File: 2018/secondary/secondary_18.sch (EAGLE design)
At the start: 35 parts, among them Q1 BUZ11, Q2 BUZ11

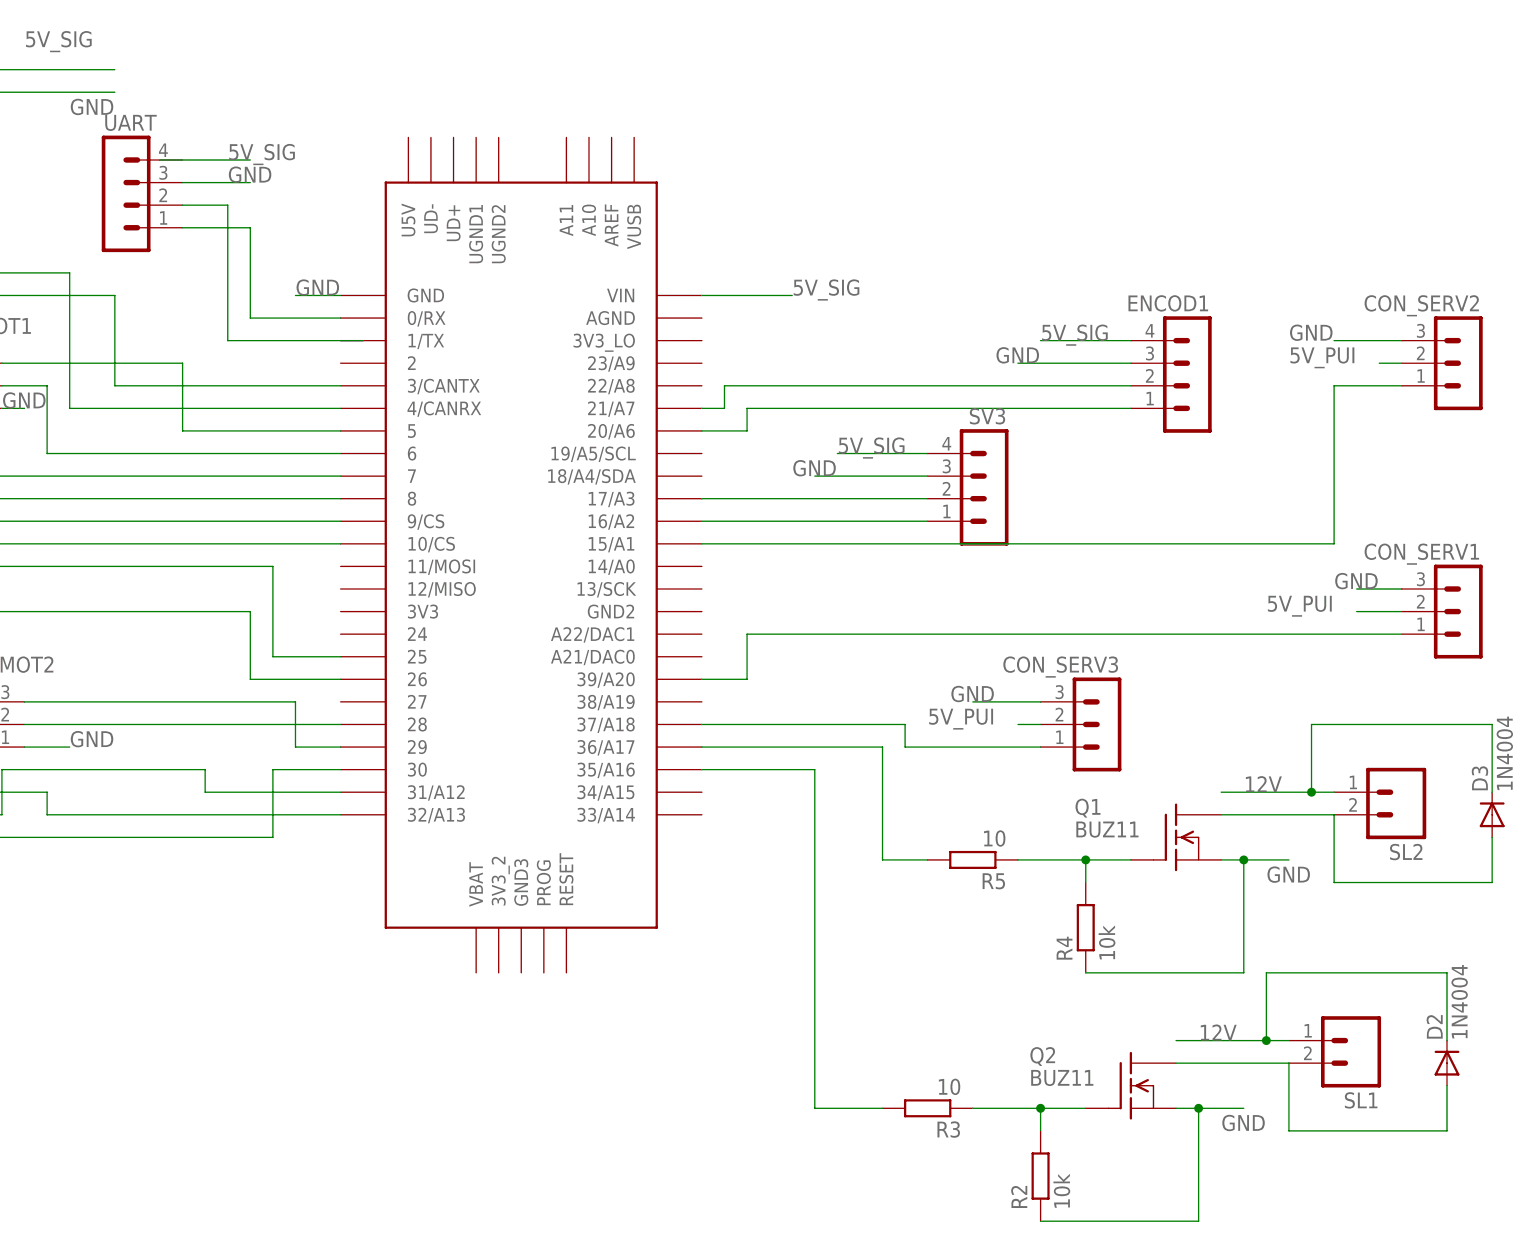
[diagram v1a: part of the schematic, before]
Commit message: [Secondary] Adds the board.
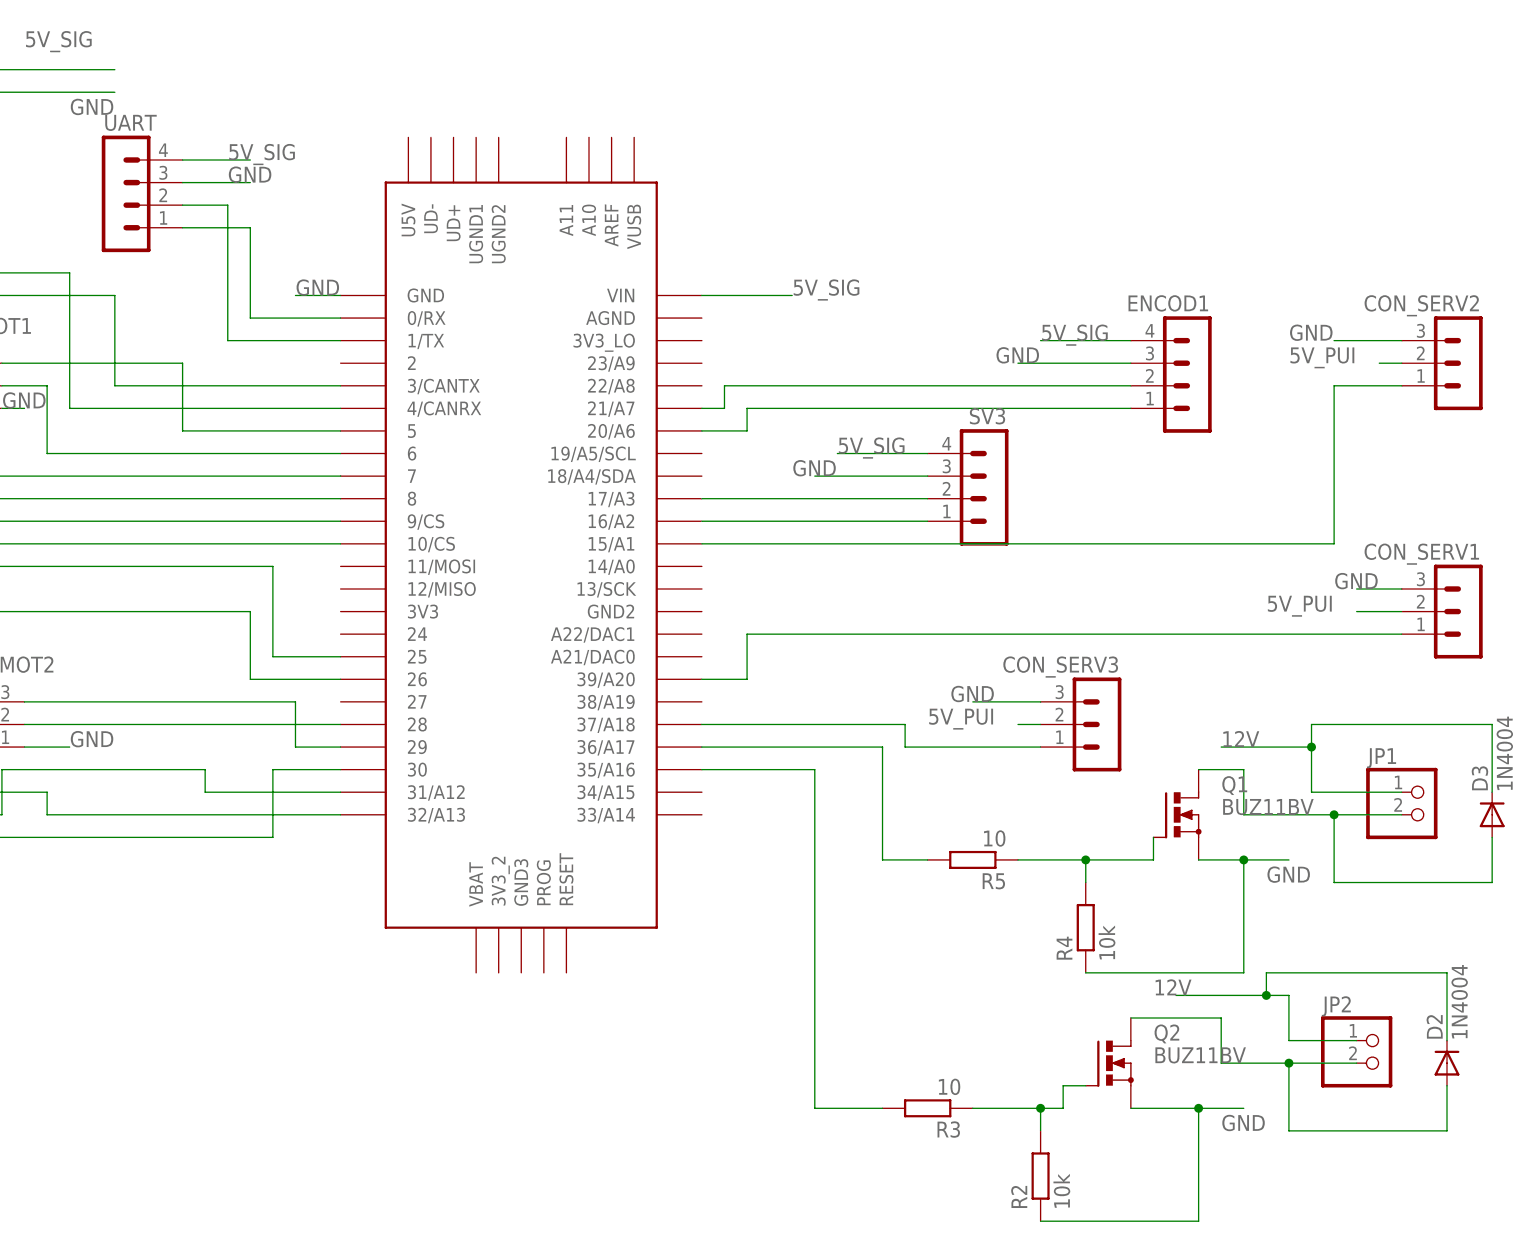
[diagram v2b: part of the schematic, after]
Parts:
- removed SL1, SL2: (no value), con-amp-quick:MA02
- added JP1, JP2: (no value), pinhead:PINHD-1X2
- Q1, Q2: value BUZ11 -> BUZ11BV; device transistor-fet:BUZ11 -> transistor-power:BUZ11BV
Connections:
- net 12V: now also JP1.1, JP2.1; no longer SL1.1, SL2.1
- net 5V_SIG: now also UART.4
- net N$12: now also JP1.2; no longer SL2.2
- net N$26: now also U$1.1/TX
- net N$8: now also JP2.2; no longer SL1.2
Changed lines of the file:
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@@
 <part name="CON_MOT2" library="con-lstb" deviceset="MA03-1" device=""/>
 <part name="SV3" library="con-lstb" deviceset="MA04-1" device=""/>
-<part name="Q2" library="transistor-fet" deviceset="BUZ11" device=""/>
+<part name="Q2" library="transistor-power" deviceset="BUZ11" device="BV"/>
 <part name="R2" library="resistor" deviceset="R-EU_" device="0204/7" value="10k"/>
 <part name="R3" library="resistor" deviceset="R-EU_" device="0204/7" value="10"/>
-<part name="SL1" library="con-amp-quick" deviceset="MA02" device=""/>
 <part name="D2" library="diode" deviceset="1N4004" device=""/>
-<part name="Q1" library="transistor-fet" deviceset="BUZ11" device=""/>
+<part name="Q1" library="transistor-power" deviceset="BUZ11" device="BV"/>
 <part name="R4" library="resistor" deviceset="R-EU_" device="0204/7" value="10k"/>
 <part name="R5" library="resistor" deviceset="R-EU_" device="0204/7" value="10"/>
-<part name="SL2" library="con-amp-quick" deviceset="MA02" device=""/>
 <part name="D3" library="diode" deviceset="1N4004" device=""/>
 <part name="ENCOD1" library="con-lstb" deviceset="MA04-1" device=""/>
@@
 <part name="UART" library="con-lstb" deviceset="MA04-1" device=""/>
 <part name="SV1" library="con-lstb" deviceset="MA06-1" device=""/>
+<part name="JP1" library="pinhead" deviceset="PINHD-1X2" device=""/>
+<part name="JP2" library="pinhead" deviceset="PINHD-1X2" device=""/>
 </parts>
 <sheets>
@@
 <instance part="CON_MOT2" gate="G$1" x="20.32" y="25.4"/>
 <instance part="SV3" gate="1" x="137.16" y="53.34" rot="MR0"/>
-<instance part="Q2" gate="G$1" x="152.4" y="-15.24"/>
+<instance part="Q2" gate="1" x="149.86" y="-12.7"/>
 <instance part="R2" gate="G$1" x="142.24" y="-25.4" rot="R90"/>
 <instance part="R3" gate="G$1" x="129.54" y="-17.78" rot="R180"/>
-<instance part="SL1" gate="G$1" x="177.8" y="-10.16" rot="R180"/>
 <instance part="D2" gate="1" x="187.96" y="-12.7" rot="R90"/>
-<instance part="Q1" gate="G$1" x="157.48" y="12.7"/>
+<instance part="Q1" gate="1" x="157.48" y="15.24"/>
 <instance part="R4" gate="G$1" x="147.32" y="2.54" rot="R90"/>
 <instance part="R5" gate="G$1" x="134.62" y="10.16" rot="R180"/>
-<instance part="SL2" gate="G$1" x="182.88" y="17.78" rot="R180"/>
 <instance part="D3" gate="1" x="193.04" y="15.24" rot="R90"/>
 <instance part="ENCOD1" gate="1" x="160.02" y="66.04" rot="MR0"/>
@@
 <instance part="UART" gate="1" x="38.1" y="86.36"/>
 <instance part="SV1" gate="1" x="-10.16" y="58.42"/>
+<instance part="JP1" gate="G$1" x="185.42" y="15.24"/>
+<instance part="JP2" gate="G$1" x="180.34" y="-12.7"/>
 </instances>
 <busses>
@@
 </segment>
 <segment>
-<pinref part="Q2" gate="G$1" pin="S"/>
-<wire x1="157.48" y1="-17.78" x2="160.02" y2="-17.78" width="0.1524" layer="91"/>
+<pinref part="Q2" gate="1" pin="S"/>
+<wire x1="152.4" y1="-17.78" x2="160.02" y2="-17.78" width="0.1524" layer="91"/>
 <label x="162.56" y="-20.32" size="1.778" layer="95"/>
 <pinref part="R2" gate="G$1" pin="1"/>
@@
 </segment>
 <segment>
-<pinref part="Q1" gate="G$1" pin="S"/>
-<wire x1="162.56" y1="10.16" x2="165.1" y2="10.16" width="0.1524" layer="91"/>
+<pinref part="Q1" gate="1" pin="S"/>
+<wire x1="160.02" y1="10.16" x2="165.1" y2="10.16" width="0.1524" layer="91"/>
 <label x="167.64" y="7.62" size="1.778" layer="95"/>
 <pinref part="R4" gate="G$1" pin="1"/>
@@
 </segment>
 <segment>
-<label x="160.02" y="-10.16" size="1.778" layer="95"/>
+<label x="154.94" y="-5.08" size="1.778" layer="95"/>
 <pinref part="D2" gate="1" pin="C"/>
-<wire x1="167.64" y1="-10.16" x2="157.48" y2="-10.16" width="0.1524" layer="91"/>
+<wire x1="167.64" y1="-5.08" x2="157.48" y2="-5.08" width="0.1524" layer="91"/>
 <wire x1="187.96" y1="-10.16" x2="187.96" y2="-2.54" width="0.1524" layer="91"/>
 <wire x1="187.96" y1="-2.54" x2="167.64" y2="-2.54" width="0.1524" layer="91"/>
-<wire x1="167.64" y1="-2.54" x2="167.64" y2="-10.16" width="0.1524" layer="91"/>
-<pinref part="SL1" gate="G$1" pin="1"/>
-<wire x1="167.64" y1="-10.16" x2="170.18" y2="-10.16" width="0.1524" layer="91"/>
-<junction x="167.64" y="-10.16"/>
-</segment>
-<segment>
-<label x="165.1" y="17.78" size="1.778" layer="95"/>
+<wire x1="167.64" y1="-2.54" x2="167.64" y2="-5.08" width="0.1524" layer="91"/>
+<junction x="167.64" y="-5.08"/>
+<pinref part="JP2" gate="G$1" pin="1"/>
+<wire x1="177.8" y1="-10.16" x2="170.18" y2="-10.16" width="0.1524" layer="91"/>
+<wire x1="170.18" y1="-10.16" x2="170.18" y2="-5.08" width="0.1524" layer="91"/>
+<wire x1="170.18" y1="-5.08" x2="167.64" y2="-5.08" width="0.1524" layer="91"/>
+</segment>
+<segment>
+<label x="162.56" y="22.86" size="1.778" layer="95"/>
 <pinref part="D3" gate="1" pin="C"/>
-<wire x1="172.72" y1="17.78" x2="162.56" y2="17.78" width="0.1524" layer="91"/>
+<wire x1="172.72" y1="22.86" x2="162.56" y2="22.86" width="0.1524" layer="91"/>
 <wire x1="193.04" y1="17.78" x2="193.04" y2="25.4" width="0.1524" layer="91"/>
 <wire x1="193.04" y1="25.4" x2="172.72" y2="25.4" width="0.1524" layer="91"/>
-<wire x1="172.72" y1="25.4" x2="172.72" y2="17.78" width="0.1524" layer="91"/>
-<pinref part="SL2" gate="G$1" pin="1"/>
-<wire x1="175.26" y1="17.78" x2="172.72" y2="17.78" width="0.1524" layer="91"/>
-<junction x="172.72" y="17.78"/>
+<wire x1="172.72" y1="25.4" x2="172.72" y2="22.86" width="0.1524" layer="91"/>
+<junction x="172.72" y="22.86"/>
+<pinref part="JP1" gate="G$1" pin="1"/>
+<wire x1="182.88" y1="17.78" x2="172.72" y2="17.78" width="0.1524" layer="91"/>
+<wire x1="172.72" y1="17.78" x2="172.72" y2="22.86" width="0.1524" layer="91"/>
 </segment>
 <segment>
@@
 </segment>
 <segment>
-<wire x1="43.18" y1="88.9" x2="53.34" y2="88.9" width="0.1524" layer="91"/>
 <label x="50.8" y="88.9" size="1.778" layer="95"/>
+<pinref part="UART" gate="1" pin="4"/>
+<wire x1="45.72" y1="88.9" x2="53.34" y2="88.9" width="0.1524" layer="91"/>
 </segment>
 <segment>
@@
 <segment>
 <pinref part="R3" gate="G$1" pin="1"/>
-<pinref part="Q2" gate="G$1" pin="G"/>
+<pinref part="Q2" gate="1" pin="G"/>
 <wire x1="134.62" y1="-17.78" x2="142.24" y2="-17.78" width="0.1524" layer="91"/>
 <pinref part="R2" gate="G$1" pin="2"/>
-<wire x1="142.24" y1="-17.78" x2="147.32" y2="-17.78" width="0.1524" layer="91"/>
+<wire x1="142.24" y1="-17.78" x2="144.78" y2="-17.78" width="0.1524" layer="91"/>
+<wire x1="144.78" y1="-17.78" x2="144.78" y2="-15.24" width="0.1524" layer="91"/>
+<wire x1="144.78" y1="-15.24" x2="147.32" y2="-15.24" width="0.1524" layer="91"/>
 <wire x1="142.24" y1="-20.32" x2="142.24" y2="-17.78" width="0.1524" layer="91"/>
 <junction x="142.24" y="-17.78"/>
@@
 <net name="N$8" class="0">
 <segment>
-<pinref part="Q2" gate="G$1" pin="D"/>
-<pinref part="SL1" gate="G$1" pin="2"/>
-<wire x1="157.48" y1="-12.7" x2="170.18" y2="-12.7" width="0.1524" layer="91"/>
+<pinref part="Q2" gate="1" pin="D"/>
+<wire x1="152.4" y1="-7.62" x2="162.56" y2="-7.62" width="0.1524" layer="91"/>
+<wire x1="162.56" y1="-7.62" x2="162.56" y2="-12.7" width="0.1524" layer="91"/>
+<wire x1="162.56" y1="-12.7" x2="170.18" y2="-12.7" width="0.1524" layer="91"/>
 <wire x1="170.18" y1="-12.7" x2="170.18" y2="-20.32" width="0.1524" layer="91"/>
 <pinref part="D2" gate="1" pin="A"/>
 <wire x1="170.18" y1="-20.32" x2="187.96" y2="-20.32" width="0.1524" layer="91"/>
 <wire x1="187.96" y1="-20.32" x2="187.96" y2="-15.24" width="0.1524" layer="91"/>
+<pinref part="JP2" gate="G$1" pin="2"/>
+<wire x1="177.8" y1="-12.7" x2="170.18" y2="-12.7" width="0.1524" layer="91"/>
+<junction x="170.18" y="-12.7"/>
 </segment>
 </net>
@@
 <segment>
 <pinref part="R5" gate="G$1" pin="1"/>
-<pinref part="Q1" gate="G$1" pin="G"/>
+<pinref part="Q1" gate="1" pin="G"/>
 <wire x1="139.7" y1="10.16" x2="147.32" y2="10.16" width="0.1524" layer="91"/>
 <pinref part="R4" gate="G$1" pin="2"/>
-<wire x1="147.32" y1="10.16" x2="152.4" y2="10.16" width="0.1524" layer="91"/>
+<wire x1="147.32" y1="10.16" x2="154.94" y2="10.16" width="0.1524" layer="91"/>
+<wire x1="154.94" y1="10.16" x2="154.94" y2="12.7" width="0.1524" layer="91"/>
 <wire x1="147.32" y1="7.62" x2="147.32" y2="10.16" width="0.1524" layer="91"/>
 <junction x="147.32" y="10.16"/>
@@
 <net name="N$12" class="0">
 <segment>
-<pinref part="Q1" gate="G$1" pin="D"/>
-<pinref part="SL2" gate="G$1" pin="2"/>
-<wire x1="162.56" y1="15.24" x2="175.26" y2="15.24" width="0.1524" layer="91"/>
+<pinref part="Q1" gate="1" pin="D"/>
+<wire x1="160.02" y1="20.32" x2="165.1" y2="20.32" width="0.1524" layer="91"/>
+<wire x1="165.1" y1="20.32" x2="165.1" y2="15.24" width="0.1524" layer="91"/>
+<wire x1="165.1" y1="15.24" x2="175.26" y2="15.24" width="0.1524" layer="91"/>
 <wire x1="175.26" y1="15.24" x2="175.26" y2="7.62" width="0.1524" layer="91"/>
 <pinref part="D3" gate="1" pin="A"/>
 <wire x1="175.26" y1="7.62" x2="193.04" y2="7.62" width="0.1524" layer="91"/>
 <wire x1="193.04" y1="7.62" x2="193.04" y2="12.7" width="0.1524" layer="91"/>
+<pinref part="JP1" gate="G$1" pin="2"/>
+<wire x1="182.88" y1="15.24" x2="175.26" y2="15.24" width="0.1524" layer="91"/>
+<junction x="175.26" y="15.24"/>
 </segment>
 </net>
@@
 <wire x1="45.72" y1="83.82" x2="50.8" y2="83.82" width="0.1524" layer="91"/>
 <wire x1="50.8" y1="83.82" x2="50.8" y2="68.58" width="0.1524" layer="91"/>
-<wire x1="50.8" y1="68.58" x2="66.04" y2="68.58" width="0.1524" layer="91"/>
-</segment>
-</net>
+<pinref part="U$1" gate="G$1" pin="1/TX"/>
+<wire x1="50.8" y1="68.58" x2="63.5" y2="68.58" width="0.1524" layer="91"/>
+</segment>
+</net>
